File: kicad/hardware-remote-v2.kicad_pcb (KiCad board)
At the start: 2 copper layers, 130 x 70 mm, 29 parts, among them J1 Flash, J2 TFT, J3 5VIN, J4 3.3VIN, J5 Conn_02x08_Odd_Even, Q1 2N7002, SW1 ANALOG_LEFT, SW2 ANALOG_RIGHT, U1 ESP32-WROOM-32E-8MB, U2 AMS1117-3.3, U3 CH343G

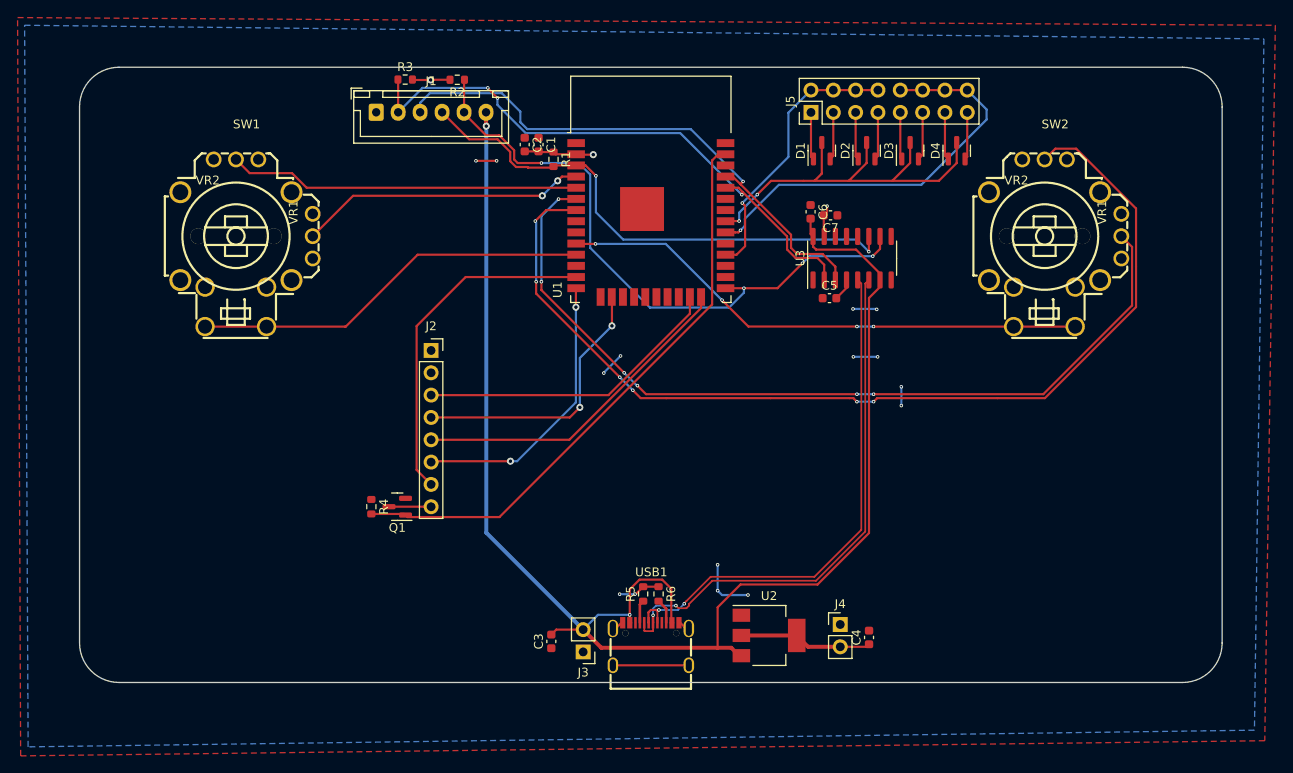
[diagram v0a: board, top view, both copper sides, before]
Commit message: Fixed DRC
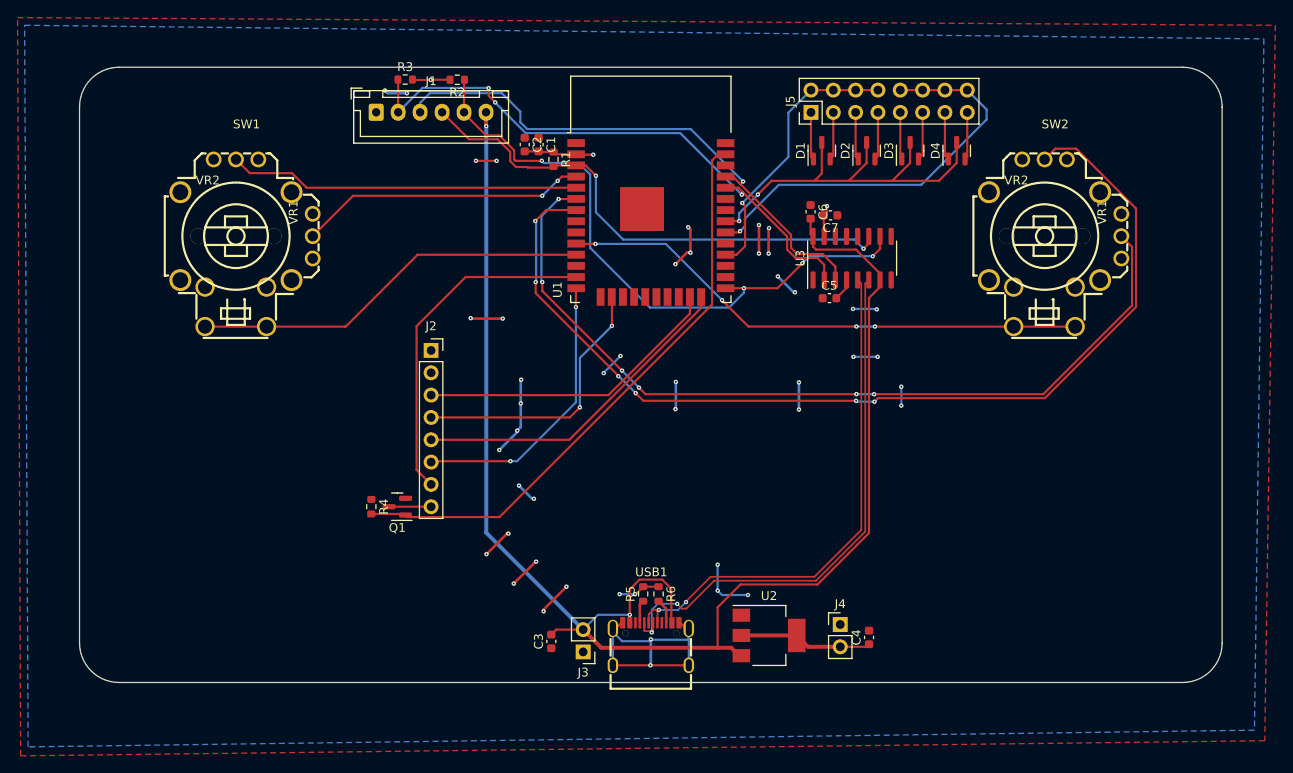
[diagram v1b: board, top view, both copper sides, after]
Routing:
- net GND: track 32.9 -> 80.8 mm, vias 13 -> 31
- net +3V3: track 33.8 -> 57.0 mm, vias 5 -> 18
- net USB_DN: track 61.4 -> 63.9 mm
- net EN: track 60.1 -> 59.3 mm
